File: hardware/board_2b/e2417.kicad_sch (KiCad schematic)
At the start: 21 parts, among them J10 CF35242D0RE-NH, Q2 SSM3K336R,LF, U16 SN74LVC1T45DCK, U27 SN74LVC2T45DCUR, U28 SN74LVC2T45DCUR, U29 SN74LVC2T45DCUR

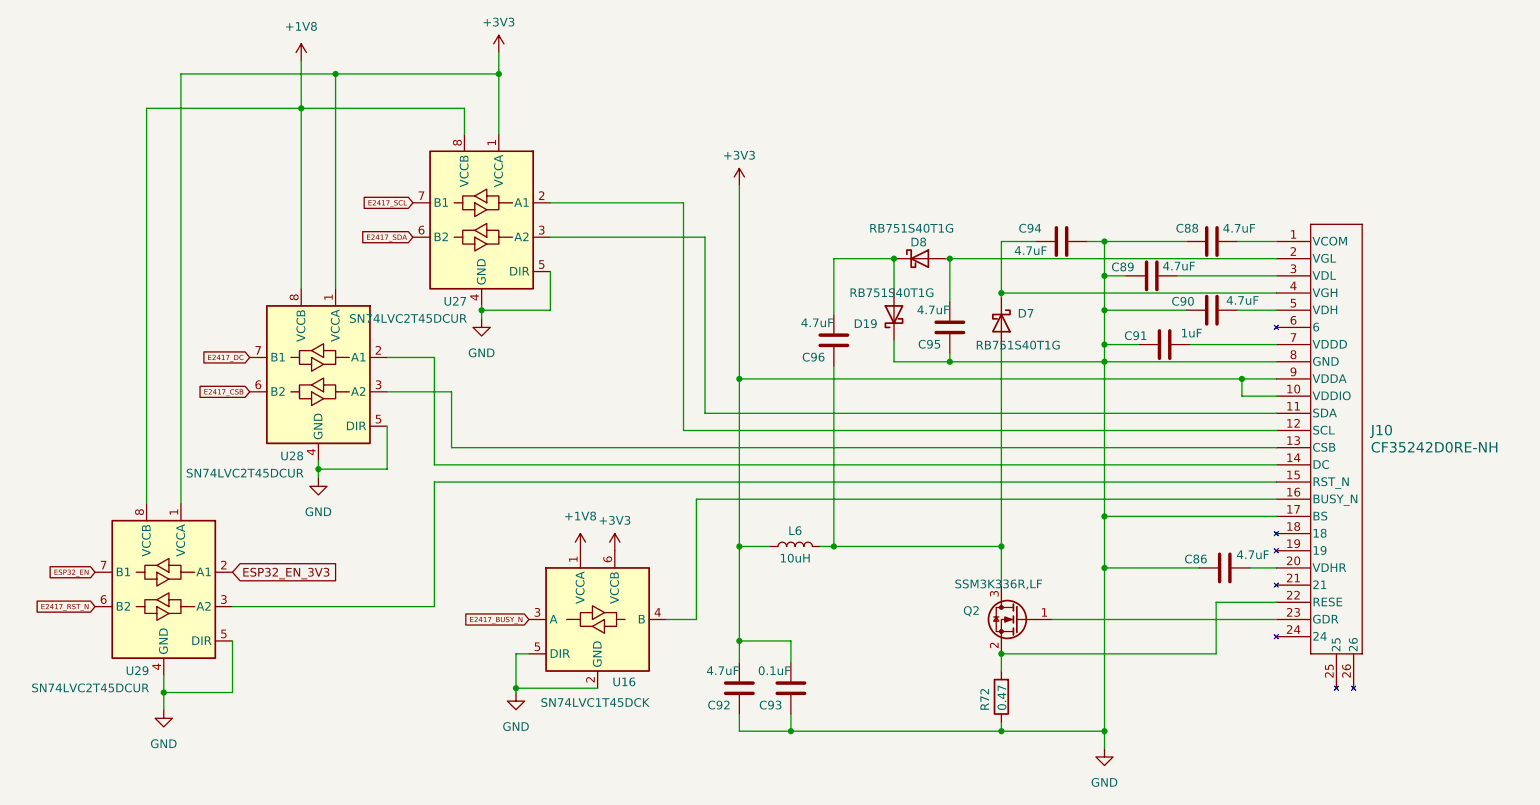
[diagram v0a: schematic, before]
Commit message: Update hardware/board_2b
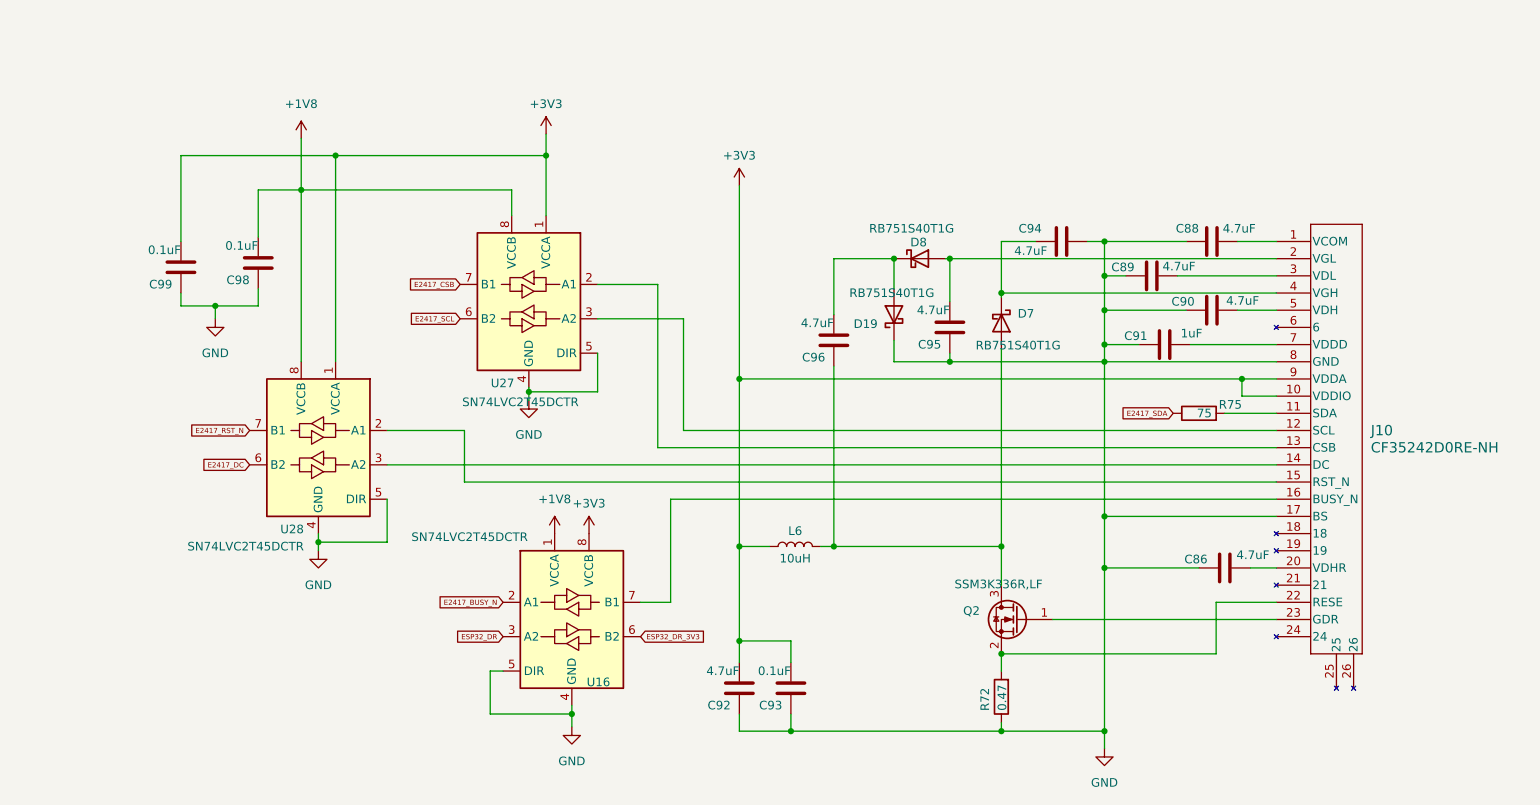
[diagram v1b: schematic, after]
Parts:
- removed U29: SN74LVC2T45DCUR, Package_SO:VSSOP-8_2.3x2mm_P0.5mm, symbol Logic_LevelTranslator:SN74LVC2T45DCUR
- added C98, C99: 0.1uF, Capacitor_SMD:C_0603_1608Metric, symbol Device:C
- added R75: 75, Resistor_SMD:R_0603_1608Metric, symbol Device:R
- U16: value SN74LVC1T45DCK -> SN74LVC2T45DCTR; footprint Package_TO_SOT_SMD:SOT-363_SC-70-6 -> Package_SO:MSOP-8_3x3mm_P0.65mm; symbol Logic_LevelTranslator:SN74LVC1T45DCK -> Logic_LevelTranslator:SN74LVC2T45DCUR
- U27, U28: value SN74LVC2T45DCUR -> SN74LVC2T45DCTR; footprint Package_SO:VSSOP-8_2.3x2mm_P0.5mm -> Package_SO:MSOP-8_3x3mm_P0.65mm
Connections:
- net +1V8: now also C98.2
- net +3V3: now also U16.8 (VCCB), C99.2; no longer U16.6 (VCCB)
- net E2417_BUSY_N: now also U16.2 (A1); no longer U16.3 (A)
- net E2417_CSB: now also U27.7 (B1); no longer U28.6 (B2)
- net E2417_DC: now also U28.6 (B2); no longer U28.7 (B1)
- net E2417_RST_N: now also U28.7 (B1)
- net E2417_SCL: now also U27.6 (B2); no longer U27.7 (B1)
- net E2417_SDA: now also R75.1; no longer U27.6 (B2)
- net GND: now also U16.4 (GND), C98.1, C99.1; no longer U16.2 (GND)
- net at U28.2 (A1): now also J10.15 (RST_N); no longer J10.14 (DC)
- net at U28.3 (A2): now also J10.14 (DC); no longer J10.13 (CSB)
- net at J10.11 (SDA): now also R75.2; no longer U27.3 (A2)
- net at J10.12 (SCL): now also U27.3 (A2); no longer U27.2 (A1)
- net at J10.16 (BUSY_N): now also U16.7 (B1); no longer U16.4 (B)
- new net: J10.13 (CSB), U27.2 (A1)
- new net ESP32_DR: U16.3 (A2)
- new net ESP32_DR_3V3: U16.6 (B2)
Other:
- moved on the sheet: U27, U28
